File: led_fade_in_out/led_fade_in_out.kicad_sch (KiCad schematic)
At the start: 7 parts, among them Q1 PN2222A, SW1 SW_SPST

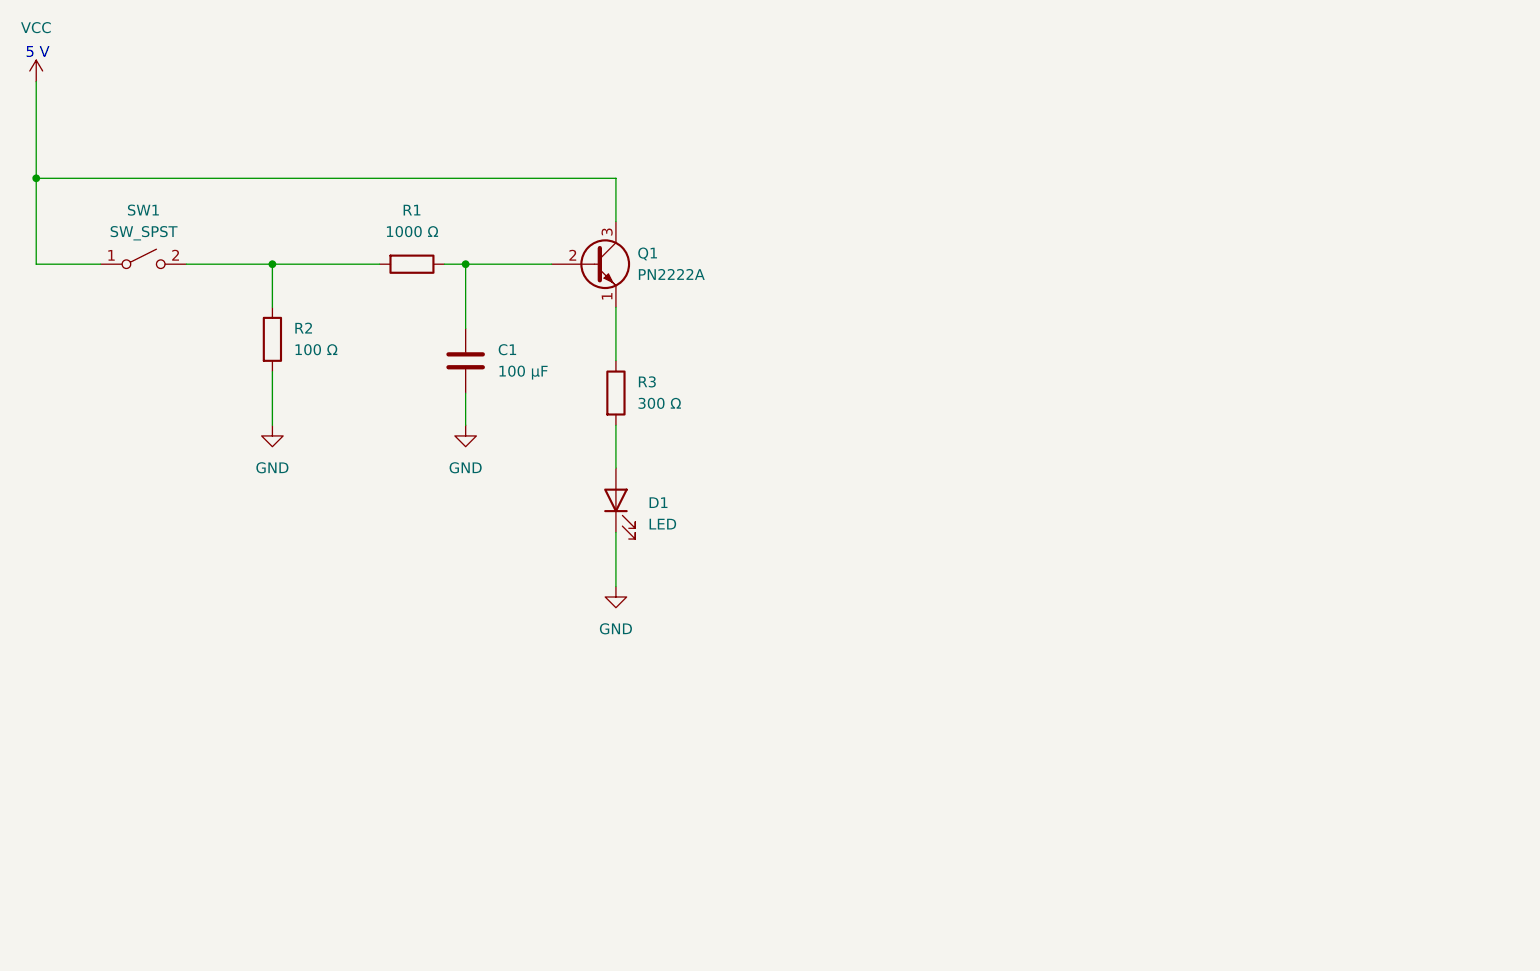
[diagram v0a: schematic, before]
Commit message: fix spacing
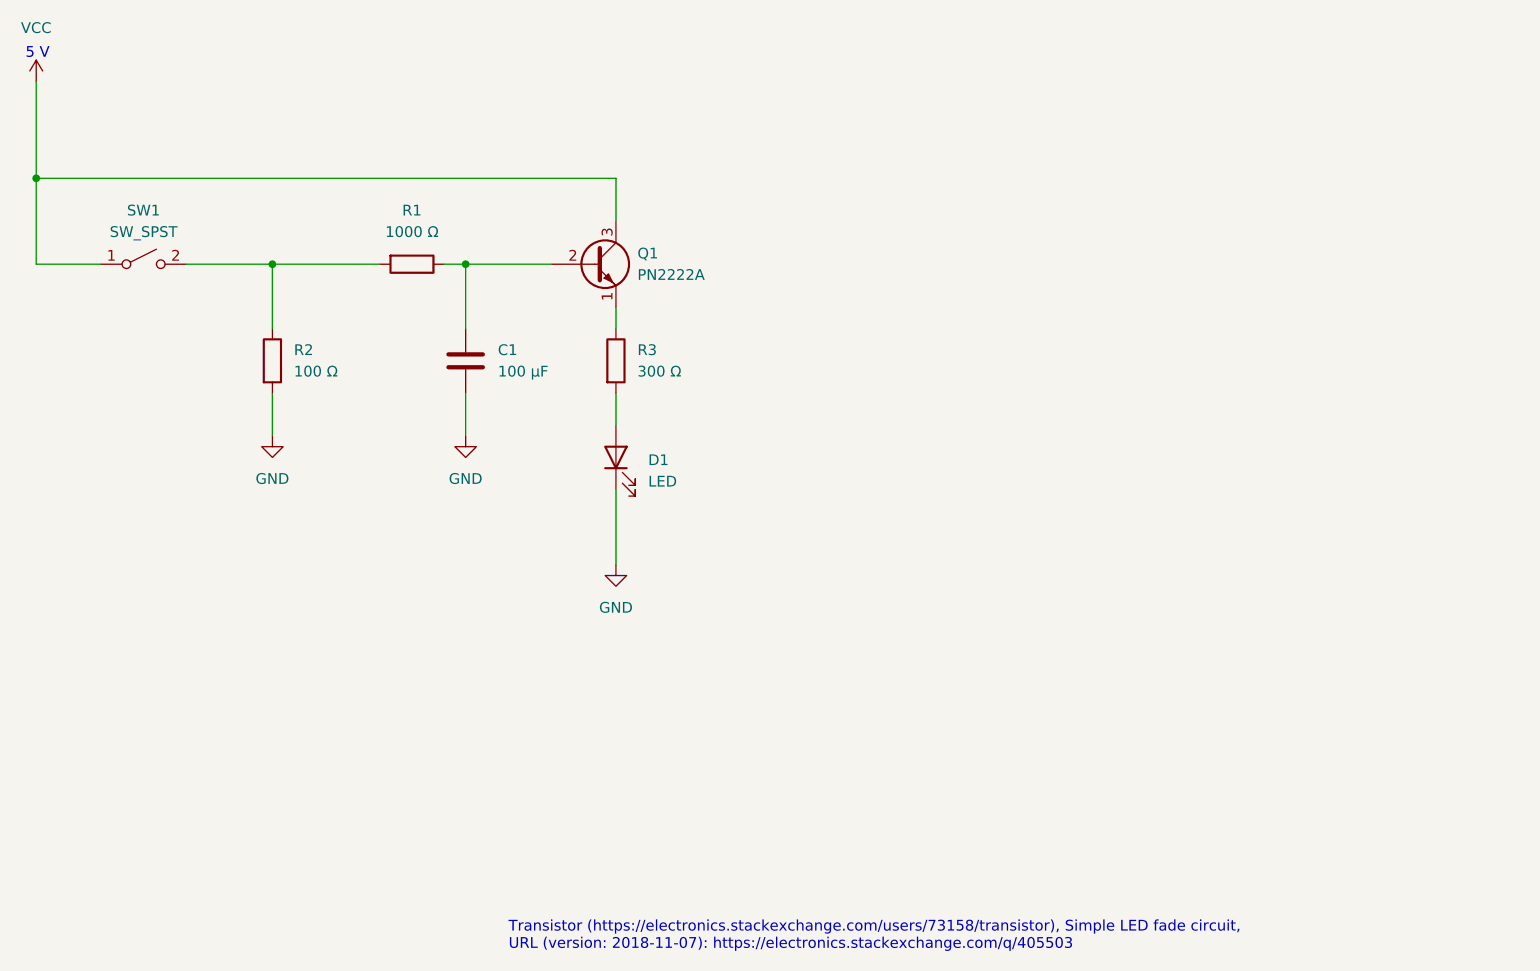
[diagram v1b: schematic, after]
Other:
- note added: "Transistor (https://electronics.stackexchange.com/users/73158/transistor), Simple LED fade circuit, URL (version: 2018-11-07): https://electronics.stackexchange.com/q/405503"
- moved on the sheet: D1, R2, R3
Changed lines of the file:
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@@
     (stroke (width 0) (type default))
   )
-  (wire (pts (xy 151.13 90.17) (xy 151.13 95.25))
+  (wire (pts (xy 151.13 90.17) (xy 151.13 97.79))
     (stroke (width 0) (type default))
   )
@@
     (stroke (width 0) (type default))
   )
-  (wire (pts (xy 151.13 102.87) (xy 151.13 109.22))
-    (stroke (width 0) (type default))
-  )
-  (wire (pts (xy 191.77 95.25) (xy 191.77 101.6))
+  (wire (pts (xy 191.77 95.25) (xy 191.77 97.79))
     (stroke (width 0) (type default))
   )
@@
     (stroke (width 0) (type default))
   )
-  (wire (pts (xy 191.77 109.22) (xy 191.77 114.3))
+  (wire (pts (xy 191.77 105.41) (xy 191.77 109.22))
     (stroke (width 0) (type default))
   )
@@
     (stroke (width 0) (type default))
   )
-  (wire (pts (xy 191.77 121.92) (xy 191.77 128.27))
+  (wire (pts (xy 191.77 116.84) (xy 191.77 125.73))
     (stroke (width 0) (type default))
   )
@@
     (stroke (width 0) (type default))
   )
-  (wire (pts (xy 173.99 109.22) (xy 173.99 105.41))
+  (wire (pts (xy 151.13 105.41) (xy 151.13 110.49))
+    (stroke (width 0) (type default))
+  )
+  (wire (pts (xy 173.99 110.49) (xy 173.99 105.41))
     (stroke (width 0) (type default))
   )
   (wire (pts (xy 123.19 68.58) (xy 123.19 80.01))
     (stroke (width 0) (type default))
+  )
+  (text "Transistor (https://electronics.stackexchange.com/users/73158/transistor), Simple LED fade circuit, \nURL (version: 2018-11-07): https://electronics.stackexchange.com/q/405503"
+    (at 179.07 171.45 0)
+    (effects (font (size 1.27 1.27)) (justify left bottom))
   )
   (text "5 V" (at 121.92 66.04 0)
     (effects (font (size 1.27 1.27)) (justify left bottom))
   )
-  (symbol (lib_id "Device:R") (at 191.77 105.41 0) (unit 1)
-    (in_bom yes) (on_board yes) (dnp no)
-    (property "Reference" "R3" (at 194.31 104.14 0)
-      (effects (font (size 1.27 1.27)) (justify left))
-    )
-    (property "Value" "300 Ω" (at 194.31 106.68 0)
-      (effects (font (size 1.27 1.27)) (justify left))
-    )
-    (property "Footprint" "" (at 189.992 105.41 90)
-      (effects (font (size 1.27 1.27)) hide)
-    )
-    (property "Datasheet" "~" (at 191.77 105.41 0)
+  (symbol (lib_id "Device:R") (at 191.77 101.6 0) (unit 1)
+    (in_bom yes) (on_board yes) (dnp no)
+    (property "Reference" "R3" (at 194.31 100.33 0)
+      (effects (font (size 1.27 1.27)) (justify left))
+    )
+    (property "Value" "300 Ω" (at 194.31 102.87 0)
+      (effects (font (size 1.27 1.27)) (justify left))
+    )
+    (property "Footprint" "" (at 189.992 101.6 90)
+      (effects (font (size 1.27 1.27)) hide)
+    )
+    (property "Datasheet" "~" (at 191.77 101.6 0)
       (effects (font (size 1.27 1.27)) hide)
     )
@@
     )
   )
-  (symbol (lib_id "power:GND") (at 151.13 109.22 0) (unit 1)
-    (in_bom yes) (on_board yes) (dnp no) (fields_autoplaced)
-    (property "Reference" "#PWR02" (at 151.13 115.57 0)
-      (effects (font (size 1.27 1.27)) hide)
-    )
-    (property "Value" "GND" (at 151.13 114.3 0)
-      (effects (font (size 1.27 1.27)))
-    )
-    (property "Footprint" "" (at 151.13 109.22 0)
-      (effects (font (size 1.27 1.27)) hide)
-    )
-    (property "Datasheet" "" (at 151.13 109.22 0)
+  (symbol (lib_id "power:GND") (at 151.13 110.49 0) (unit 1)
+    (in_bom yes) (on_board yes) (dnp no) (fields_autoplaced)
+    (property "Reference" "#PWR02" (at 151.13 116.84 0)
+      (effects (font (size 1.27 1.27)) hide)
+    )
+    (property "Value" "GND" (at 151.13 115.57 0)
+      (effects (font (size 1.27 1.27)))
+    )
+    (property "Footprint" "" (at 151.13 110.49 0)
+      (effects (font (size 1.27 1.27)) hide)
+    )
+    (property "Datasheet" "" (at 151.13 110.49 0)
       (effects (font (size 1.27 1.27)) hide)
     )
@@
     )
   )
-  (symbol (lib_id "Device:LED") (at 191.77 118.11 90) (unit 1)
-    (in_bom yes) (on_board yes) (dnp no)
-    (property "Reference" "D1" (at 195.58 118.4275 90)
+  (symbol (lib_id "Device:LED") (at 191.77 113.03 90) (unit 1)
+    (in_bom yes) (on_board yes) (dnp no)
+    (property "Reference" "D1" (at 195.58 113.3475 90)
       (effects (font (size 1.27 1.27)) (justify right))
     )
-    (property "Value" "LED" (at 195.58 120.9675 90)
+    (property "Value" "LED" (at 195.58 115.8875 90)
       (effects (font (size 1.27 1.27)) (justify right))
     )
-    (property "Footprint" "" (at 191.77 118.11 0)
-      (effects (font (size 1.27 1.27)) hide)
-    )
-    (property "Datasheet" "~" (at 191.77 118.11 0)
+    (property "Footprint" "" (at 191.77 113.03 0)
+      (effects (font (size 1.27 1.27)) hide)
+    )
+    (property "Datasheet" "~" (at 191.77 113.03 0)
       (effects (font (size 1.27 1.27)) hide)
     )
@@
     )
   )
-  (symbol (lib_id "power:GND") (at 173.99 109.22 0) (unit 1)
-    (in_bom yes) (on_board yes) (dnp no) (fields_autoplaced)
-    (property "Reference" "#PWR04" (at 173.99 115.57 0)
-      (effects (font (size 1.27 1.27)) hide)
-    )
-    (property "Value" "GND" (at 173.99 114.3 0)
-      (effects (font (size 1.27 1.27)))
-    )
-    (property "Footprint" "" (at 173.99 109.22 0)
-      (effects (font (size 1.27 1.27)) hide)
-    )
-    (property "Datasheet" "" (at 173.99 109.22 0)
+  (symbol (lib_id "power:GND") (at 173.99 110.49 0) (unit 1)
+    (in_bom yes) (on_board yes) (dnp no) (fields_autoplaced)
+    (property "Reference" "#PWR04" (at 173.99 116.84 0)
+      (effects (font (size 1.27 1.27)) hide)
+    )
+    (property "Value" "GND" (at 173.99 115.57 0)
+      (effects (font (size 1.27 1.27)))
+    )
+    (property "Footprint" "" (at 173.99 110.49 0)
+      (effects (font (size 1.27 1.27)) hide)
+    )
+    (property "Datasheet" "" (at 173.99 110.49 0)
       (effects (font (size 1.27 1.27)) hide)
     )
@@
     )
   )
-  (symbol (lib_id "Device:R") (at 151.13 99.06 0) (unit 1)
-    (in_bom yes) (on_board yes) (dnp no) (fields_autoplaced)
-    (property "Reference" "R2" (at 153.67 97.79 0)
-      (effects (font (size 1.27 1.27)) (justify left))
-    )
-    (property "Value" "100 Ω" (at 153.67 100.33 0)
-      (effects (font (size 1.27 1.27)) (justify left))
-    )
-    (property "Footprint" "" (at 149.352 99.06 90)
-      (effects (font (size 1.27 1.27)) hide)
-    )
-    (property "Datasheet" "~" (at 151.13 99.06 0)
+  (symbol (lib_id "Device:R") (at 151.13 101.6 0) (unit 1)
+    (in_bom yes) (on_board yes) (dnp no) (fields_autoplaced)
+    (property "Reference" "R2" (at 153.67 100.33 0)
+      (effects (font (size 1.27 1.27)) (justify left))
+    )
+    (property "Value" "100 Ω" (at 153.67 102.87 0)
+      (effects (font (size 1.27 1.27)) (justify left))
+    )
+    (property "Footprint" "" (at 149.352 101.6 90)
+      (effects (font (size 1.27 1.27)) hide)
+    )
+    (property "Datasheet" "~" (at 151.13 101.6 0)
       (effects (font (size 1.27 1.27)) hide)
     )
@@
     )
   )
-  (symbol (lib_id "power:GND") (at 191.77 128.27 0) (unit 1)
-    (in_bom yes) (on_board yes) (dnp no) (fields_autoplaced)
-    (property "Reference" "#PWR03" (at 191.77 134.62 0)
-      (effects (font (size 1.27 1.27)) hide)
-    )
-    (property "Value" "GND" (at 191.77 133.35 0)
-      (effects (font (size 1.27 1.27)))
-    )
-    (property "Footprint" "" (at 191.77 128.27 0)
-      (effects (font (size 1.27 1.27)) hide)
-    )
-    (property "Datasheet" "" (at 191.77 128.27 0)
-      (effects (font (size 1.27 1.27)) hide)
-    )
+  (symbol (lib_id "power:GND") (at 191.77 125.73 0) (unit 1)
+    (in_bom yes) (on_board yes) (dnp no) (fields_autoplaced)
+    (property "Reference" "#PWR03" (at 191.77 132.08 0)
+      (effects (font (size 1.27 1.27)) hide)
+    )
+    (property "Value" "GND" (at 191.77 130.81 0)
+      (effects (font (size 1.27 1.27)))
+    )
+    (property "Footprint" "" (at 191.77 125.73 0)
+      (effects (font (size 1.27 1.27)) hide)
+    )
+    (property "Datasheet" "" (at 191.77 125.73 0)
+      (effects (font (size 1.27 1.27)) hide)
+    )
